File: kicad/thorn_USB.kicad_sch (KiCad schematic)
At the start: 7 parts, among them J1 Conn_01x04, J2 USB_C_Receptacle_USB2.0_14P, U2 NCP1117-3.3_SOT223

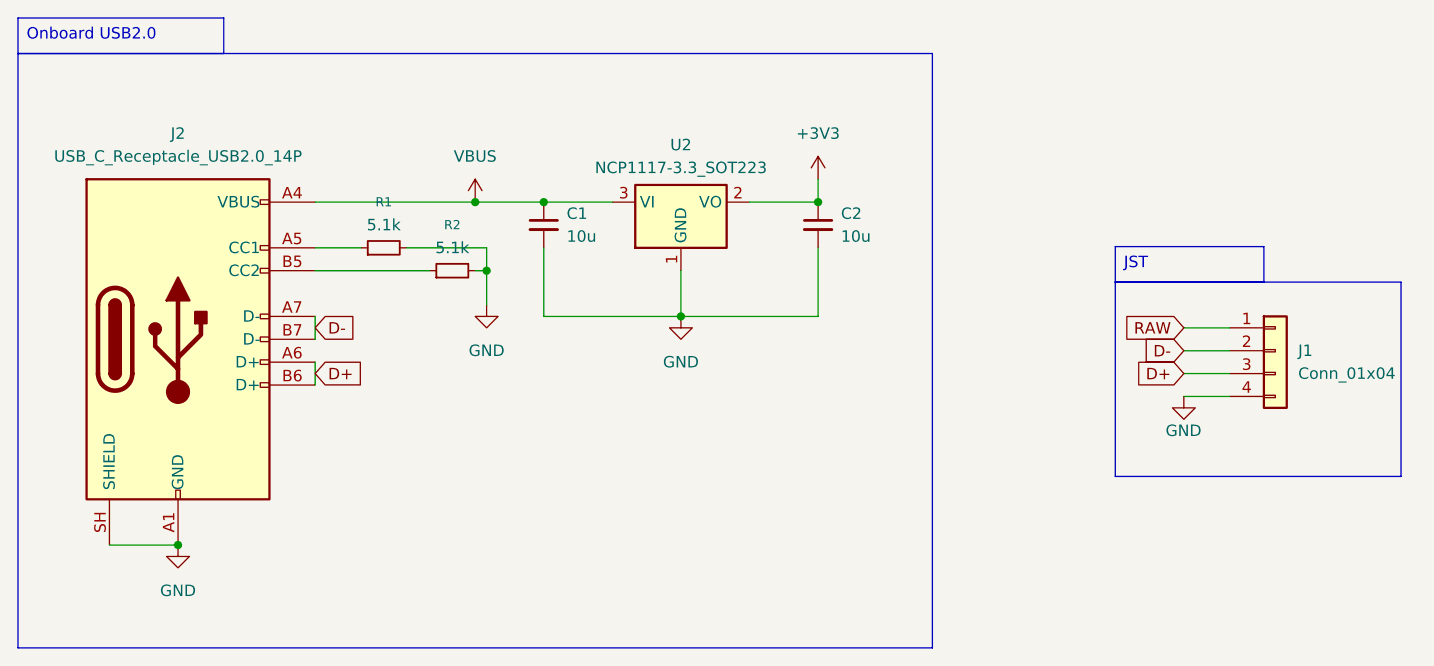
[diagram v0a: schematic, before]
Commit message: feat: finished preliminary wiring
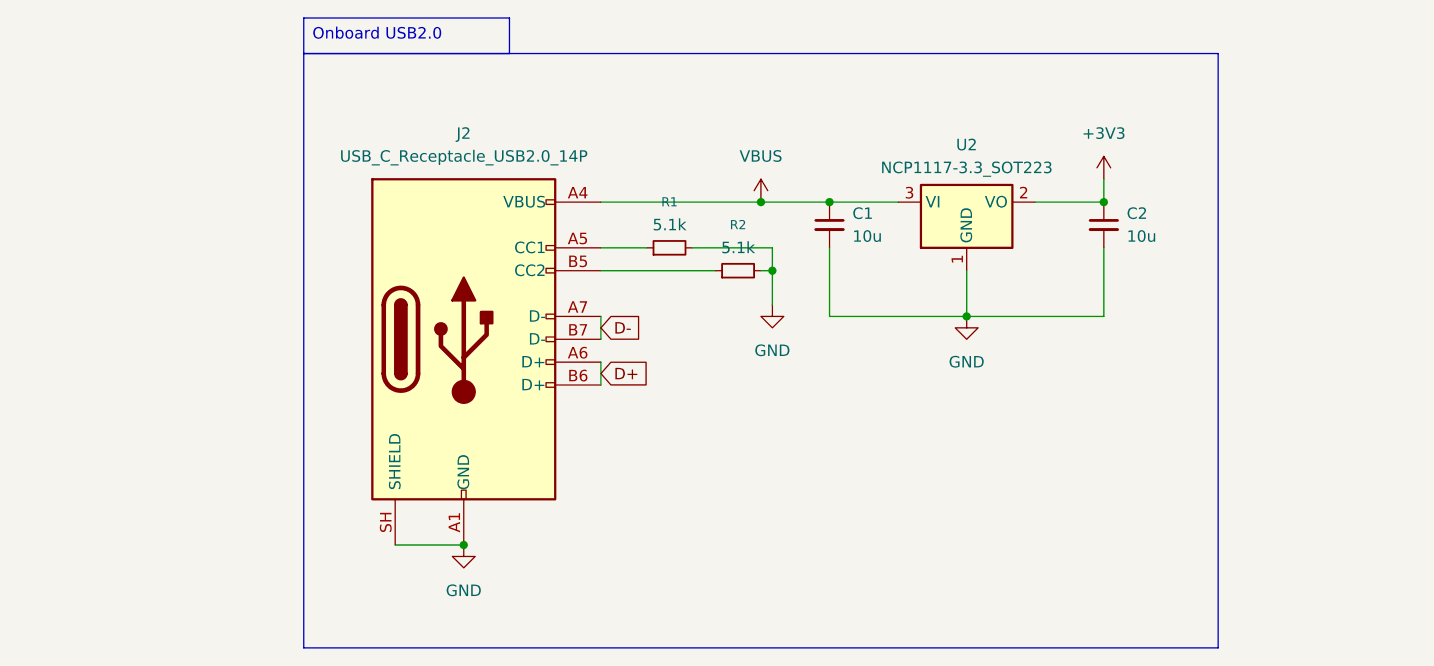
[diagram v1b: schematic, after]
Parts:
- removed J1: Conn_01x04, Connector_JST:JST_SH_SM04B-SRSS-TB_1x04-1MP_P1.00mm_Horizontal, symbol Connector_Generic:Conn_01x04
- J2: footprint Connector_USB:USB_C_Receptacle_HRO_TYPE-C-31-M-17 -> Connector_USB:USB_C_Receptacle_JAE_DX07S016JA1R1500
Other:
- moved on the sheet: C1, C2, J2, R1, R2, U2
